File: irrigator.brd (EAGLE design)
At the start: 79.7 x 47 mm, 27 parts, among them IC1 MEGA8-AI, IC2 78L05Z, T1 BT136, X1 MSTBA2

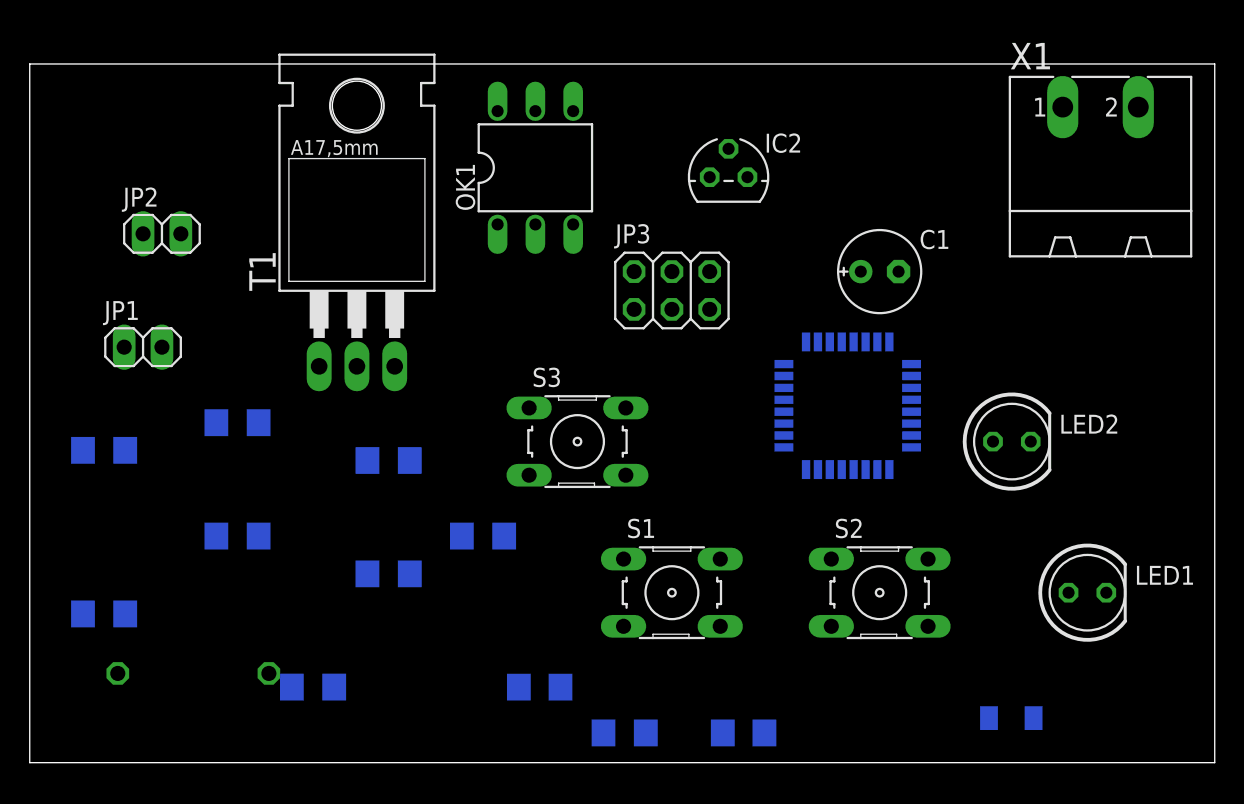
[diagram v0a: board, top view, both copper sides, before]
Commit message: fix. errors and manual routing
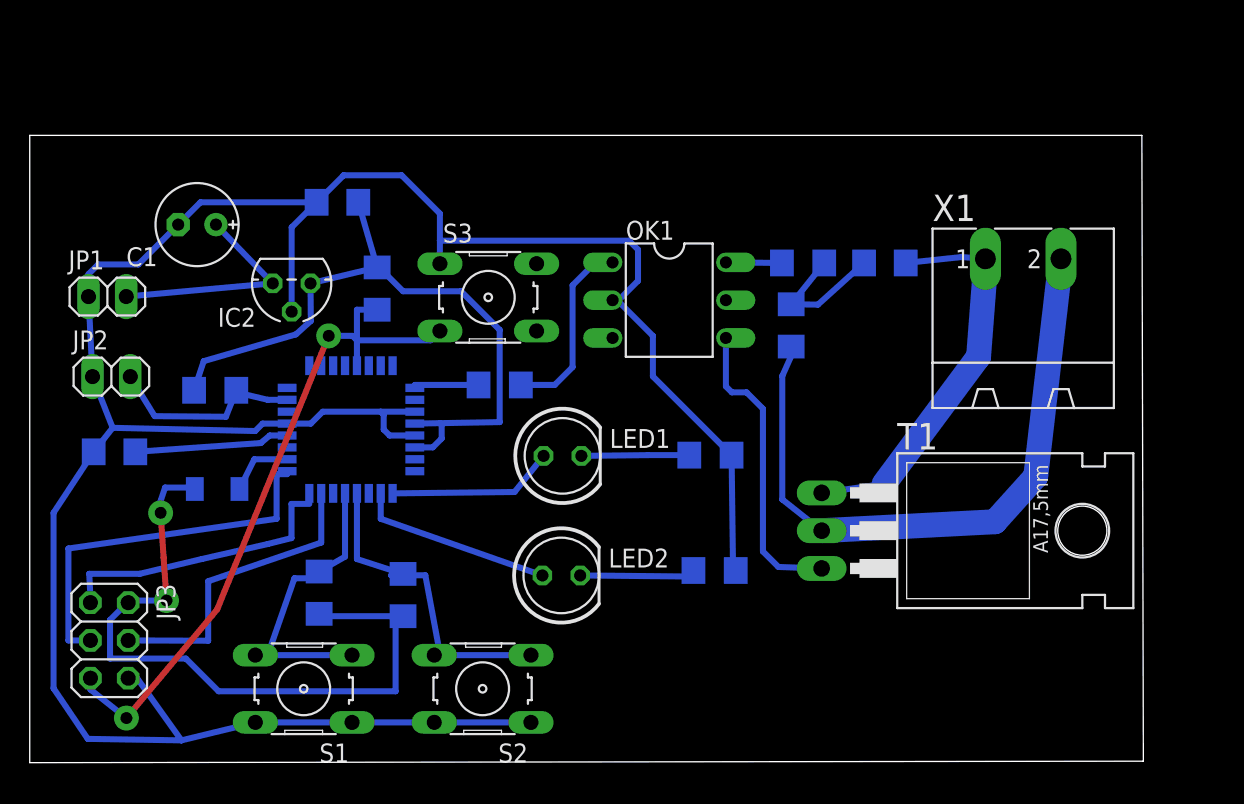
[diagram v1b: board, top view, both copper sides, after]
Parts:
- C3: device rcl:C102-054X133 -> rcl:C1206
- moved L1 55.6 mm to (12.6, 18.4), turned to 180 degrees
- moved C3 54.1 mm to (57.5, 33.6), turned to 180 degrees
- moved R8 50.1 mm to (51.2, 29.4), turned to 270 degrees
- moved R7 48.7 mm to (52.0, 33.6), turned to 180 degrees
- moved C4 46.3 mm to (5.70, 20.9)
- moved C1 46.0 mm to (11.2, 36.2), turned to 180 degrees
- moved JP3 44.6 mm to (5.35, 8.22), turned to 270 degrees
- moved T1 41.4 mm to (59.6, 15.6), turned to 270 degrees
- moved LED1 36.5 mm to (35.8, 20.6)
- moved C2 35.3 mm to (20.7, 37.7)
- moved IC1 33.4 mm to (21.6, 22.4)
- moved LED2 31.6 mm to (35.7, 12.6)
- moved IC2 30.2 mm to (17.6, 32.2), turned to 180 degrees
- moved R5 28.1 mm to (46.0, 12.9), turned to 180 degrees
- moved S2 27.5 mm to (30.4, 4.97), turned to 180 degrees
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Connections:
- new net MISO: IC1.16, JP3.1
- new net MOSI: IC1.15, JP3.4
- new net SCK: IC1.17, JP3.3
- net BUTTON_1: now also IC1.13; no longer IC1.12
- net BUTTON_2: now also IC1.12; no longer IC1.13
- net LED_1: now also IC1.9; no longer IC1.15, JP3.4
- net LED_2: now also IC1.10; no longer IC1.16, JP3.1
- net SENS_IN: no longer JP3.3
- net SW: now also IC1.1; no longer IC1.14
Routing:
- net GND: track 0.00 -> 172.2 mm
- net VCC: track 0.00 -> 94.3 mm, vias 0 -> 2
- net RESET: track 0.00 -> 46.2 mm, vias 0 -> 2
- net N$7: track 0.00 -> 44.4 mm
- net N$8: track 0.00 -> 26.8 mm
- net SCK: track 0.00 -> 25.7 mm
- net BUTTON_2: track 0.00 -> 22.7 mm
- net MOSI: track 0.00 -> 20.7 mm
- net N$6: track 0.00 -> 20.4 mm
- net BUTTON_1: track 0.00 -> 20.4 mm
- net MISO: track 0.00 -> 19.3 mm
- net VIN: track 0.00 -> 15.4 mm
- net SENS_IN: track 0.00 -> 13.4 mm
- net LED_2: track 0.00 -> 13.2 mm
- net N$1: track 0.00 -> 12.8 mm
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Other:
- board size 79.7 x 47 mm -> 74.9 x 42.2 mm
